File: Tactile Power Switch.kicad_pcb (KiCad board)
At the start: 2 copper layers, 22 x 26 mm, 18 parts, among them J1 OSTTC020162, J2 OSTTC020162, Q1 BC847B_215, Q2 BC847B_215, Q4 NDT2955, SW1 SW_SPST

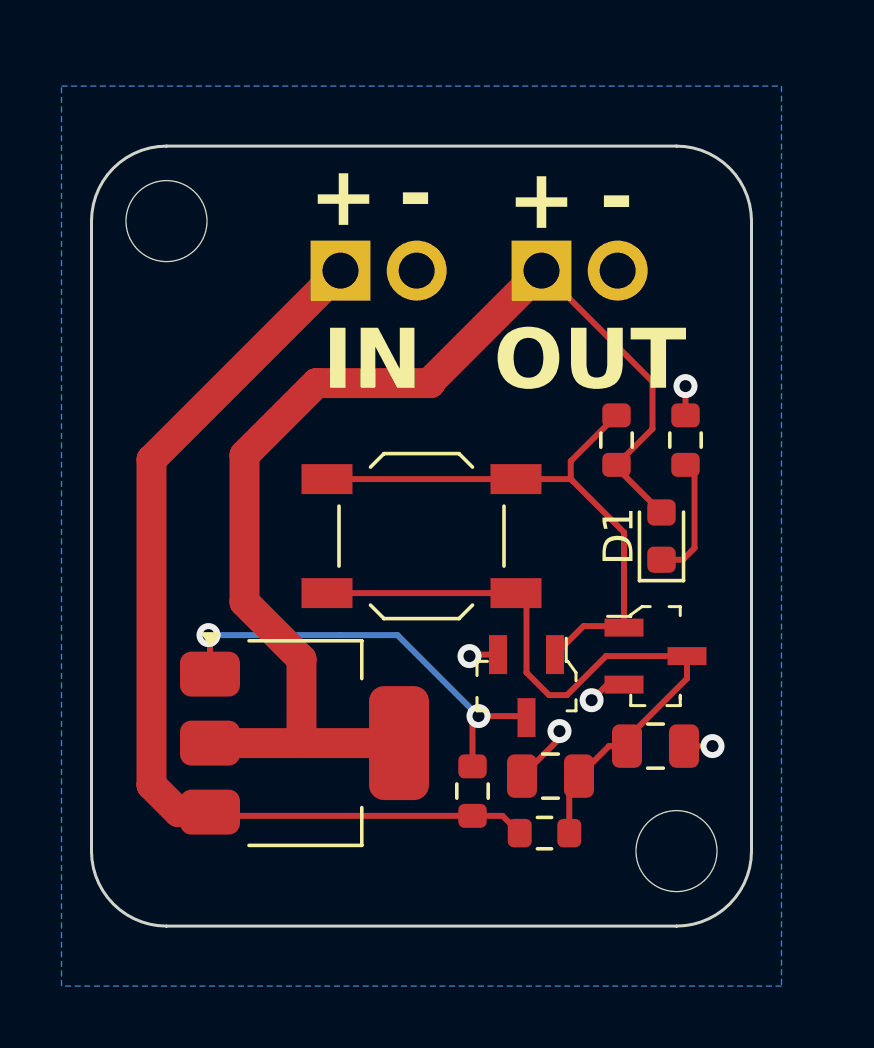
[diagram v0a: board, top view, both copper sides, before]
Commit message: mfg file initiated
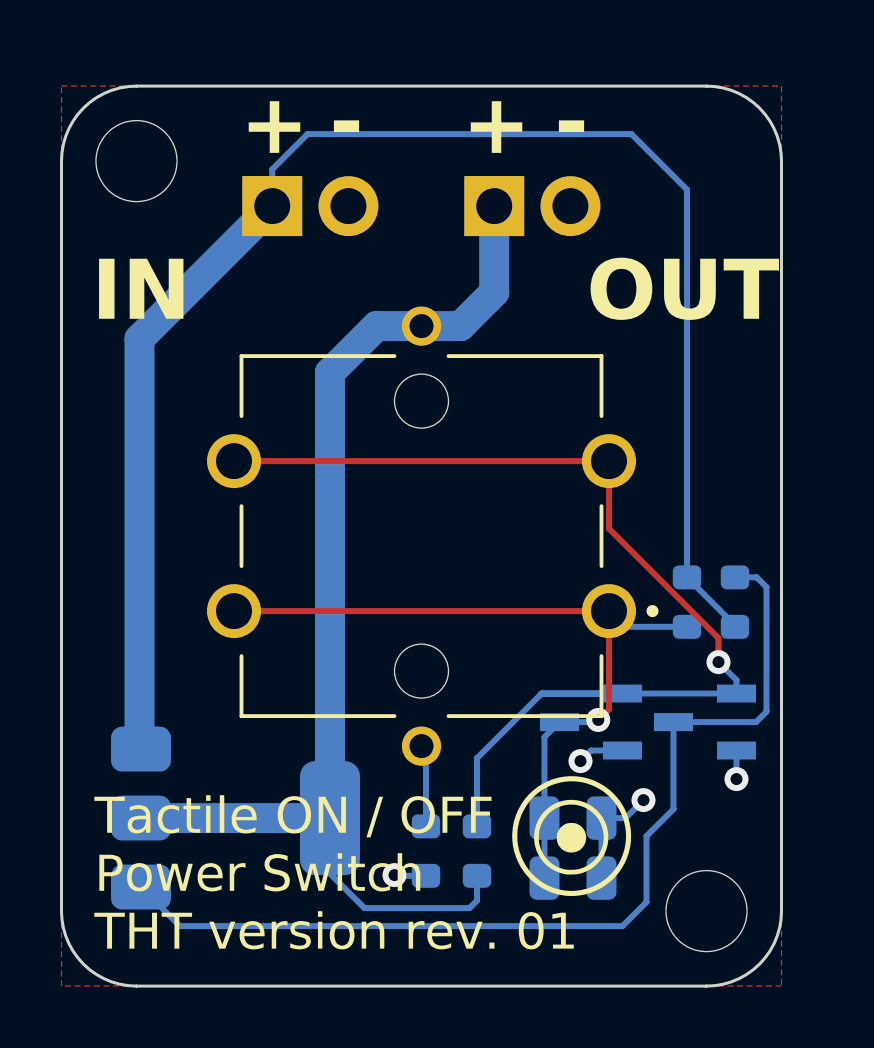
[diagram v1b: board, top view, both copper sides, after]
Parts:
- removed D1: GREEN, LED_SMD:LED_0603_1608Metric
- removed REF**: OSHW-Symbol_6.7x6mm_SilkScreen, Symbol:OSHW-Symbol_6.7x6mm_SilkScreen
- removed SW1: SW_SPST, Button_Switch_SMD:SW_SPST_TL3342
- added S1: TSD1265, SW_TSD1265:SW_TSD1265, F.Cu at (120.0, 59.0)
- C1, C2, Q1, Q2, Q4, R1, R2, R3, R4: moved to B.Cu
- G***: moved to F.Cu
- moved R4 16.2 mm to (120.2, 69.5), turned to -90 degrees
- moved G*** 15.2 mm to (125.0, 69.0), turned to 0 degrees
- moved R2 14.5 mm to (121.8, 69.5)
- moved R1 10.8 mm to (130.4, 61.2)
- moved G*** 9.65 mm to (120.2, 59.0)
- moved R3 9.05 mm to (128.8, 61.2), turned to -90 degrees
- moved Q1 6.07 mm to (129.4, 65.2), turned to 180 degrees
- moved C1 3.65 mm to (125.0, 68.4)
- moved C2 3.48 mm to (125.0, 70.4), turned to 0 degrees
- moved Q4 3.40 mm to (113.8, 68.4)
- moved J1 3.13 mm to (115.0, 48.0)
- moved Q2 3.08 mm to (125.7, 65.2), turned to 180 degrees
- moved J2 2.67 mm to (122.4, 48.0)
- moved H1 2.24 mm to (129.5, 71.5)
- moved H2 2.24 mm to (110.5, 46.5)
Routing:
- net +12V: track 32.7 -> 51.5 mm
- net Net-(Q1-C): track 14.8 -> 32.7 mm, vias 2 -> 0
- net Net-(Q1-B): track 19.3 -> 36.5 mm, vias 0 -> 1
- net Net-(Q2-C): track 23.2 -> 25.8 mm, vias 0 -> 1
- net Net-(R4-Pad1): track 4.16 -> 2.74 mm
- net VDD: track 39.9 -> 38.8 mm
- net GND: track 6.21 -> 7.20 mm, vias 5 -> 4
- added copper zone on F.Cu, net GND
- removed copper zone on B.Cu, net GND
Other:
- board size 22 x 26 mm -> 24 x 30 mm
- board text added: "Tactile ON / OFF Power Switch THT version rev. 01"
- board text removed: "SMD VERSION REV.01"
- board text removed: "Tactile ON/OFF Power Button"
